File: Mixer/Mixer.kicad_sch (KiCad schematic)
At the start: 28 parts, among them J1 Conn_01x06_Male, Q1 BC547, Q2 BC557, U1 TL072, U2 Aux_flush, U3 Aux_flush, U4 Aux_flush, U5 Aux_flush, U6 Aux_flush

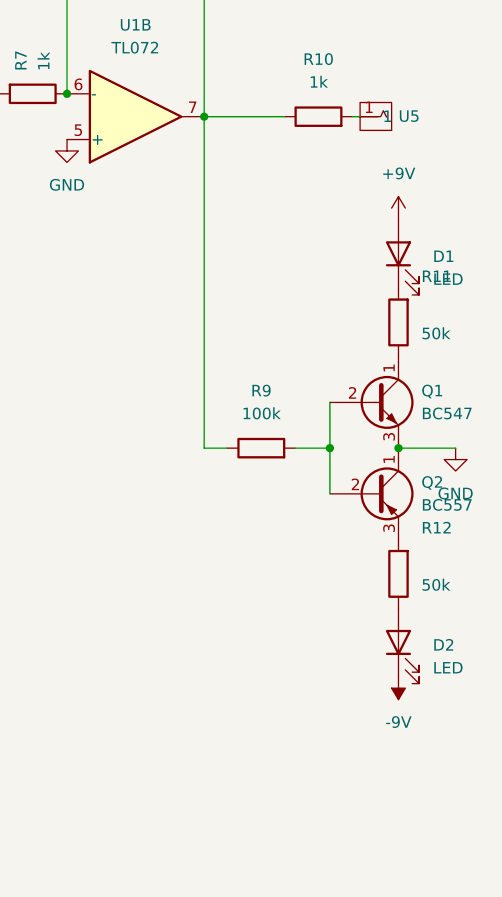
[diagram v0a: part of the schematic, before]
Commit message: Add files via upload
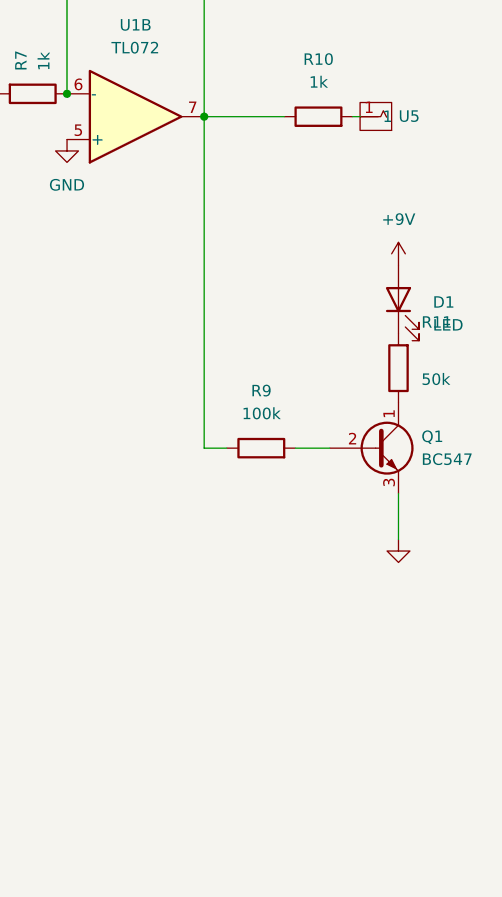
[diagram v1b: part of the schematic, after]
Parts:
- removed D2: LED, LED_THT:LED_D5.0mm, symbol Device:LED
- removed Q2: BC557, Package_TO_SOT_THT:TO-92_Inline_Wide, symbol Transistor_BJT:BC557
- removed R12: 50k, Resistor_THT:R_Axial_DIN0204_L3.6mm_D1.6mm_P7.62mm_Horizontal, symbol Device:R
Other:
- moved on the sheet: D1, Q1, R11
